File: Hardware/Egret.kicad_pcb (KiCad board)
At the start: 2 copper layers, 64.6 x 60.3 mm, 60 parts, among them Q1 S8050, Q2 S8050, Q3 AO3415AL, SW1 TD-1106SN-5.0H-160, SW2 TD-1106SN-5.0H-160, U1 WS2812B-B, U10 ST7789_FPC_PAD, U2 AN2051-245_2.4G, U3 ESP32--PICO--D4, U4 MPU6050-YJLTY, U5 AMS1117-3.3, U6 BH1750FVI-TR, U7 CP2102N-A02-GQFN28, U8 FPC-SMD_8P-P0.5, U9 FPC-SMD_8P-P0.5

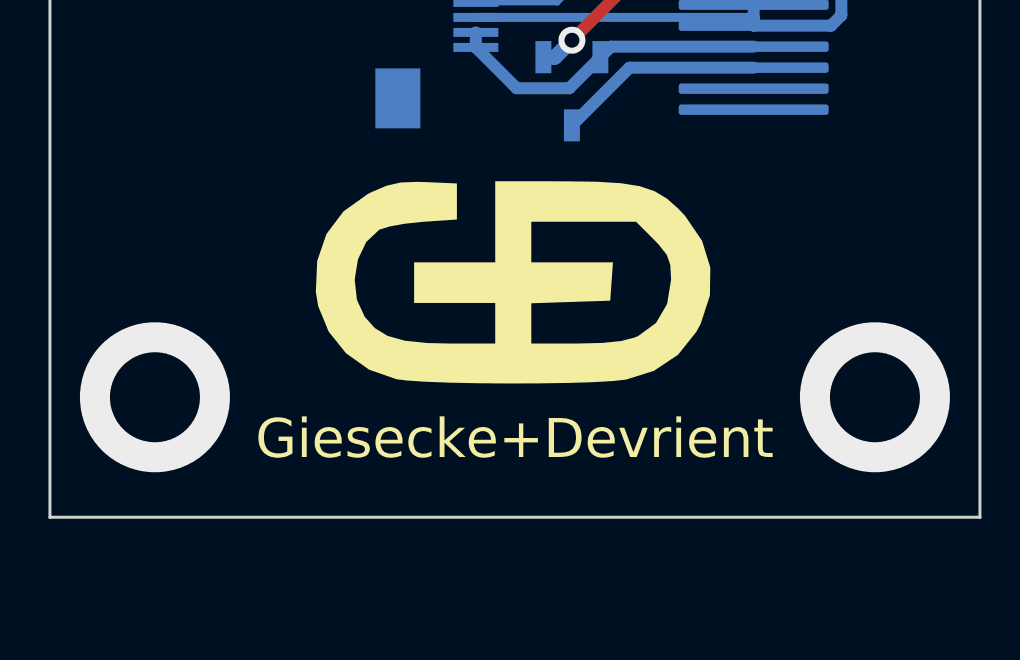
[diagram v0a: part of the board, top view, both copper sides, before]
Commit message: update
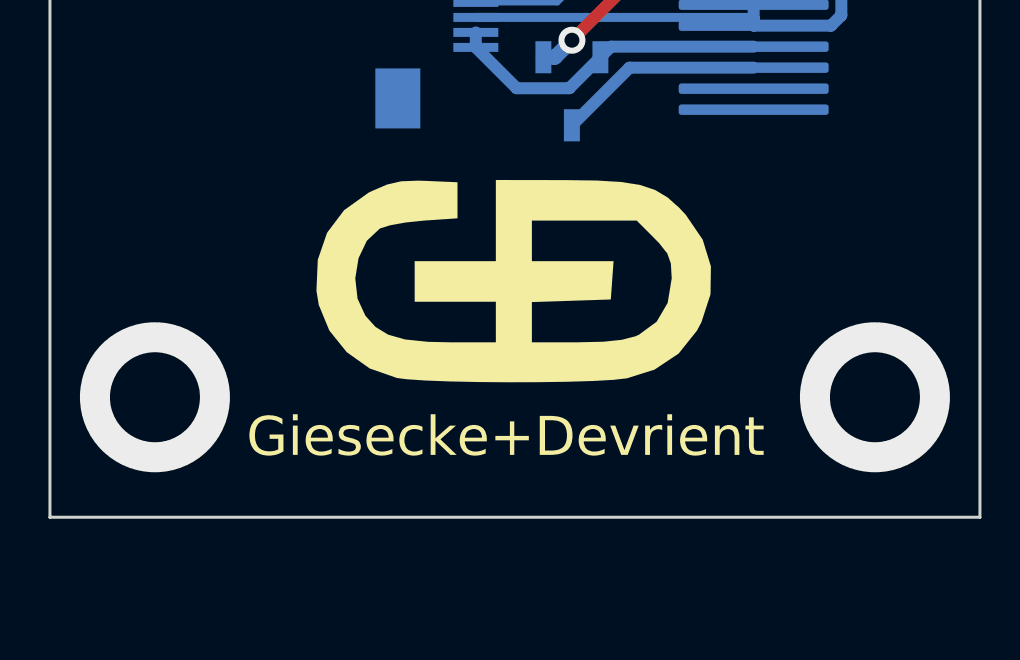
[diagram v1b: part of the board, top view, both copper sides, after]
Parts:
- moved ? 0.20 mm to (166.3, 87.0)
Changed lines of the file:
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@@
   )
   (footprint "Uinika.Footprint:G+D-big" (layer "F.Cu")
-    (at 148.273859 125.145001)
+    (at 148.293859 125.105001)
     (attr board_only exclude_from_pos_files exclude_from_bom)
     (fp_text reference "" (at 0 0) (layer "F.SilkS")
@@
   )
   (footprint "Uinika.Footprint:G+D-big" (layer "B.Cu")
-    (at 148.23 125.13 180)
+    (at 148.25 125.09 180)
     (attr board_only exclude_from_pos_files exclude_from_bom)
     (fp_text reference "" (at 0 0) (layer "B.SilkS")
@@
   )
   (footprint "Uinika.Footprint:G+D-big" (layer "B.Cu")
-    (at 166.304999 87.196141 -90)
+    (at 166.3 87 -90)
     (attr board_only exclude_from_pos_files exclude_from_bom)
     (fp_text reference "" (at 0 0 90) (layer "B.SilkS")
@@
     (effects (font (size 0.5 0.5) (thickness 0.1)) (justify mirror))
   )
-  (gr_text "Giesecke+Devrient" (at 171.29 86.63 90) (layer "B.SilkS")
+  (gr_text "Giesecke+Devrient" (at 171.6 86.63 90) (layer "B.SilkS")
     (effects (font (size 1.3 1.3) (thickness 0.2)) (justify mirror))
   )
@@
     (effects (font (size 0.5 0.5) (thickness 0.1)) (justify mirror))
   )
-  (gr_text "Giesecke+Devrient" (at 148.35 130.41) (layer "B.SilkS")
+  (gr_text "Giesecke+Devrient" (at 148.62 130.36) (layer "B.SilkS")
     (effects (font (size 1.3 1.3) (thickness 0.2)) (justify mirror))
   )
@@
     (effects (font (size 0.5 0.5) (thickness 0.1)))
   )
-  (gr_text "Giesecke+Devrient" (at 148.32 130.43) (layer "F.SilkS")
+  (gr_text "Giesecke+Devrient" (at 148.02 130.36) (layer "F.SilkS")
     (effects (font (size 1.3 1.3) (thickness 0.2)))
   )
